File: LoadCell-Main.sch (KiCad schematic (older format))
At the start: 47 parts, among them J1 M20-8760242, J2 0.100_1X4, J3 M20-8760242, J4 0.100_1X4, J5 M20-8760242, J6 0.100_1X4, J7 M20-8760242, J8 0.100_1X4, U1 L78L12ABUTR, U2 LM321SN3T1G, U3 L78L12ABUTR, U4 LM321SN3T1G, U5 L78L12ABUTR, U6 LM321SN3T1G, U7 L78L12ABUTR, U8 LM321SN3T1G

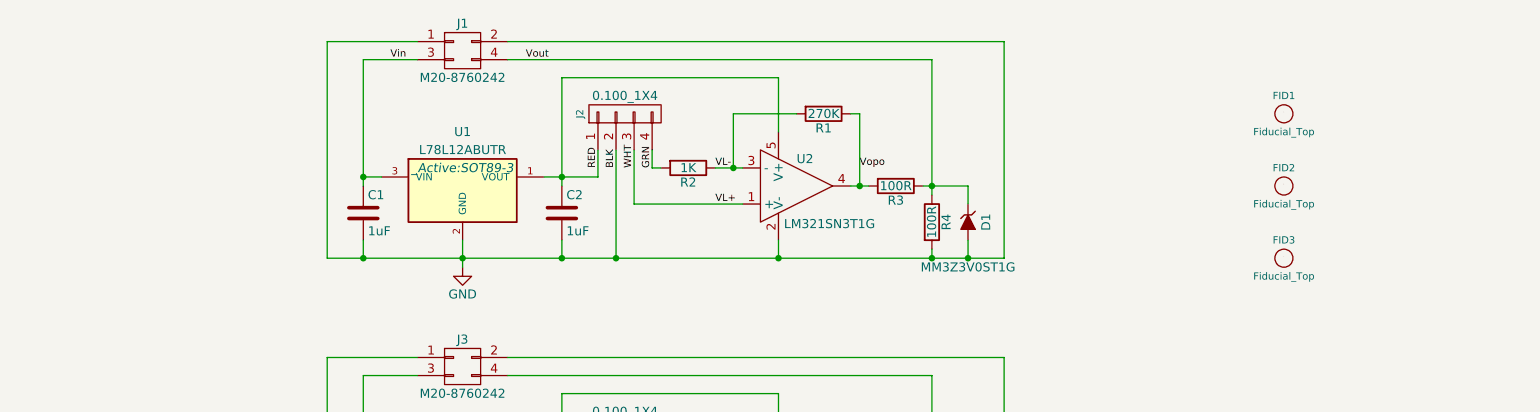
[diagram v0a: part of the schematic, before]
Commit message: Started changes the version 2
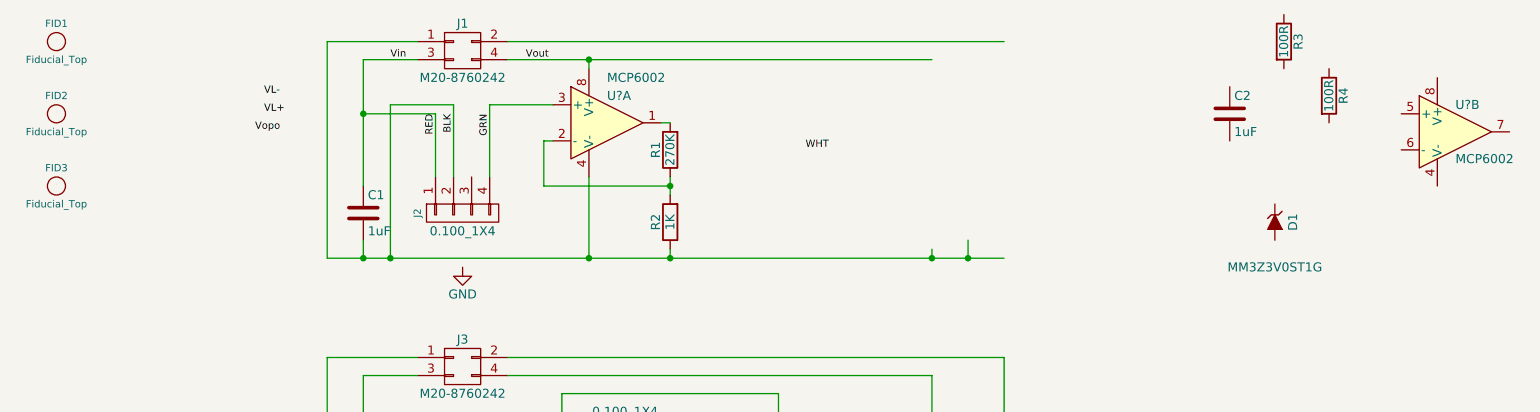
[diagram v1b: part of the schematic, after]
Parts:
- removed U1: L78L12ABUTR, _Active:SOT89-3, symbol L78L12ABUTR
- removed U2: LM321SN3T1G, _Active:SOT-23-5, symbol LM321_23-5
- added U? (x2): MCP6002, symbol MCP6002
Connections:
- wire segments 136 -> 127
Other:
- moved on the sheet: C2, D1, FID1, FID2, FID3, J2, R1, R2, R3, R4
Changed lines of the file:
@@
 L C C2
 U 1 1 5A80CCD0
-P 3850 1750
-F 0 "C2" H 3875 1850 50  0000 L CNN
-F 1 "1uF" H 3875 1650 50  0000 L CNN
-F 2 "_Passive:C_0402" H 3888 1600 50  0001 C CNN
-F 3 "" H 3850 1750 50  0000 C CNN
-	1    3850 1750
+P 7550 1200
+F 0 "C2" H 7575 1300 50  0000 L CNN
+F 1 "1uF" H 7575 1100 50  0000 L CNN
+F 2 "_Passive:C_0402" H 7588 1050 50  0001 C CNN
+F 3 "" H 7550 1200 50  0000 C CNN
+	1    7550 1200
 	1    0    0    -1
 $EndComp
@@
 L R R4
 U 1 1 5A80CD03
-P 5900 1800
-F 0 "R4" V 5980 1800 50  0000 C CNN
-F 1 "100R" V 5900 1800 50  0000 C CNN
-F 2 "_Passive:R_0402" V 5830 1800 50  0001 C CNN
-F 3 "" H 5900 1800 50  0000 C CNN
-	1    5900 1800
-	1    0    0    -1
-$EndComp
-$Comp
-L L78L12ABUTR U1
-U 1 1 5A80CDDA
-P 3300 1600
-F 0 "U1" H 3300 1900 50  0000 C CNN
-F 1 "L78L12ABUTR" H 3300 1800 50  0000 C CNN
-F 2 "_Active:SOT89-3" H 3300 1700 50  0000 C CIN
-F 3 "" H 3300 1600 50  0000 C CNN
-	1    3300 1600
+P 8100 1100
+F 0 "R4" V 8180 1100 50  0000 C CNN
+F 1 "100R" V 8100 1100 50  0000 C CNN
+F 2 "_Passive:R_0402" V 8030 1100 50  0001 C CNN
+F 3 "" H 8100 1100 50  0000 C CNN
+	1    8100 1100
 	1    0    0    -1
 $EndComp
@@
 L R R3
 U 1 1 5A80EB34
-P 5700 1600
-F 0 "R3" V 5780 1600 50  0000 C CNN
-F 1 "100R" V 5700 1600 50  0000 C CNN
-F 2 "_Passive:R_0402" V 5630 1600 50  0001 C CNN
-F 3 "" H 5700 1600 50  0000 C CNN
-	1    5700 1600
-	0    1    1    0
+P 7850 800
+F 0 "R3" V 7930 800 50  0000 C CNN
+F 1 "100R" V 7850 800 50  0000 C CNN
+F 2 "_Passive:R_0402" V 7780 800 50  0001 C CNN
+F 3 "" H 7850 800 50  0000 C CNN
+	1    7850 800
+	1    0    0    -1
 $EndComp
 $Comp
@@
 L R R1
 U 1 1 5A80EC35
-P 5300 1200
-F 0 "R1" V 5380 1200 50  0000 C CNN
-F 1 "270K" V 5300 1200 50  0000 C CNN
-F 2 "_Passive:R_0402" V 5230 1200 50  0001 C CNN
-F 3 "" H 5300 1200 50  0000 C CNN
-	1    5300 1200
-	0    1    1    0
+P 4450 1400
+F 0 "R1" V 4530 1400 50  0000 C CNN
+F 1 "270K" V 4450 1400 50  0000 C CNN
+F 2 "_Passive:R_0402" V 4380 1400 50  0001 C CNN
+F 3 "" H 4450 1400 50  0000 C CNN
+	1    4450 1400
+	-1   0    0    1
 $EndComp
 $Comp
 L R R2
 U 1 1 5A80EC7B
-P 4550 1500
-F 0 "R2" V 4630 1500 50  0000 C CNN
-F 1 "1K" V 4550 1500 50  0000 C CNN
-F 2 "_Passive:R_0402" V 4480 1500 50  0001 C CNN
-F 3 "" H 4550 1500 50  0000 C CNN
-	1    4550 1500
-	0    1    1    0
-$EndComp
-$Comp
-L LM321_23-5 U2
-U 1 1 5A80F3F0
-P 5150 1600
-F 0 "U2" H 5150 1750 50  0000 L CNN
-F 1 "LM321SN3T1G" H 5080 1390 50  0000 L CNN
-F 2 "_Active:SOT-23-5" H 5150 1600 50  0001 C CNN
-F 3 "" H 5150 1600 50  0000 C CNN
-	1    5150 1600
-	1    0    0    -1
+P 4450 1800
+F 0 "R2" V 4530 1800 50  0000 C CNN
+F 1 "1K" V 4450 1800 50  0000 C CNN
+F 2 "_Passive:R_0402" V 4380 1800 50  0001 C CNN
+F 3 "" H 4450 1800 50  0000 C CNN
+	1    4450 1800
+	-1   0    0    1
 $EndComp
 $Comp
 L D_ZENER D1
 U 1 1 5A81D761
-P 6100 1800
-F 0 "D1" H 6100 1900 50  0000 C CNN
-F 1 "MM3Z3V0ST1G" V 6350 1800 50  0000 C CNN
-F 2 "_Passive:SOD-323" H 6100 1800 50  0001 C CNN
-F 3 "" H 6100 1800 50  0000 C CNN
-	1    6100 1800
+P 7800 1800
+F 0 "D1" H 7800 1900 50  0000 C CNN
+F 1 "MM3Z3V0ST1G" V 8050 1800 50  0000 C CNN
+F 2 "_Passive:SOD-323" H 7800 1800 50  0001 C CNN
+F 3 "" H 7800 1800 50  0000 C CNN
+	1    7800 1800
 	0    1    1    0
 $EndComp
@@
 Text Label 3650 900  0    40   ~ 0
 Vout
-Text Label 4700 1500 0    40   ~ 0
+Text Label 2200 1100 0    40   ~ 0
 VL-
-Text Label 4700 1700 0    40   ~ 0
+Text Label 2200 1200 0    40   ~ 0
 VL+
-Text Label 5500 1500 0    40   ~ 0
+Text Label 2150 1300 0    40   ~ 0
 Vopo
 $Comp
 L 0.100_1X4 J2
 U 1 1 5A85E78B
-P 4200 1200
-F 0 "J2" H 4200 1450 40  0000 C CNN
-F 1 "0.100_1X4" V 4300 1200 50  0000 C CNN
-F 2 "_Connector:0.100_1x4_micro" H 4200 1200 50  0001 C CNN
-F 3 "" H 4200 1200 50  0000 C CNN
-	1    4200 1200
-	0    -1   -1   0
-$EndComp
-Text Label 4050 1500 1    40   ~ 0
+P 3300 1750
+F 0 "J2" H 3300 2000 40  0000 C CNN
+F 1 "0.100_1X4" V 3400 1750 50  0000 C CNN
+F 2 "_Connector:0.100_1x4_micro" H 3300 1750 50  0001 C CNN
+F 3 "" H 3300 1750 50  0000 C CNN
+	1    3300 1750
+	0    -1   1    0
+$EndComp
+Text Label 3150 1200 3    40   ~ 0
 RED
-Text Label 4150 1500 1    40   ~ 0
+Text Label 3250 1200 3    40   ~ 0
 BLK
-Text Label 4350 1500 1    40   ~ 0
+Text Label 3450 1200 3    40   ~ 0
 GRN
-Text Label 4250 1500 1    40   ~ 0
+Text Label 5200 1400 0    40   ~ 0
 WHT
 $Comp
@@
 Wire Wire Line
 	2750 900  2750 1600
-Connection ~ 2750 1550
-Wire Wire Line
-	4700 1500 4850 1500
-Wire Wire Line
-	5150 1200 4800 1200
-Wire Wire Line
-	4800 1200 4800 1500
-Connection ~ 4800 1500
-Wire Wire Line
-	5450 1600 5550 1600
-Wire Wire Line
-	5450 1200 5500 1200
-Wire Wire Line
-	5500 1200 5500 1600
-Connection ~ 5500 1600
-Connection ~ 5900 1600
 Connection ~ 5900 2000
 Wire Wire Line
-	5850 1600 6100 1600
-Wire Wire Line
 	2750 1900 2750 2000
 Wire Wire Line
 	5900 2000 5900 1950
 Wire Wire Line
-	6100 1600 6100 1700
-Wire Wire Line
 	6100 2000 6100 1900
 Wire Wire Line
 	3050 900  2750 900
 Wire Wire Line
-	2850 1550 2750 1550
-Wire Wire Line
 	2550 800  3050 800
-Wire Wire Line
-	3750 1550 4050 1550
-Connection ~ 3850 1550
-Wire Wire Line
-	3850 2000 3850 1900
-Wire Wire Line
-	4050 1550 4050 1400
-Wire Wire Line
-	3850 1000 3850 1600
-Wire Wire Line
-	4150 2000 4150 1400
-Wire Wire Line
-	3850 1000 5050 1000
-Wire Wire Line
-	5050 1000 5050 1300
-Wire Wire Line
-	4350 1400 4350 1500
-Wire Wire Line
-	4350 1500 4400 1500
-Wire Wire Line
-	4850 1700 4250 1700
-Wire Wire Line
-	4250 1700 4250 1400
 Wire Wire Line
 	2550 2000 6300 2000
 Connection ~ 2750 2000
 Wire Wire Line
-	3300 1900 3300 2050
-Connection ~ 3300 2000
-Connection ~ 3850 2000
-Connection ~ 4150 2000
-Wire Wire Line
-	5050 1900 5050 2000
-Connection ~ 5050 2000
-Wire Wire Line
 	3550 900  5900 900
-Wire Wire Line
-	5900 900  5900 1650
 Wire Wire Line
 	3550 800  6300 800
@@
 Wire Wire Line
 	5900 6350 5900 7100
-Wire Wire Line
-	6300 800  6300 2000
 Connection ~ 6100 2000
 Wire Wire Line
@@
 L Fiducial_Top FID1
 U 1 1 5A8C10DE
-P 7850 1200
-F 0 "FID1" H 7850 1300 40  0000 C CNN
-F 1 "Fiducial_Top" H 7850 1100 40  0000 C CNN
-F 2 "_Connector:Fiducial_0.040_Top" H 7850 1200 150 0001 C CNN
-F 3 "" H 7850 1200 150 0000 C CNN
-	1    7850 1200
+P 1050 800
+F 0 "FID1" H 1050 900 40  0000 C CNN
+F 1 "Fiducial_Top" H 1050 700 40  0000 C CNN
+F 2 "_Connector:Fiducial_0.040_Top" H 1050 800 150 0001 C CNN
+F 3 "" H 1050 800 150 0000 C CNN
+	1    1050 800
 	1    0    0    -1
 $EndComp
@@
 L Fiducial_Top FID2
 U 1 1 5A8C1162
-P 7850 1600
-F 0 "FID2" H 7850 1700 40  0000 C CNN
-F 1 "Fiducial_Top" H 7850 1500 40  0000 C CNN
-F 2 "_Connector:Fiducial_0.040_Top" H 7850 1600 150 0001 C CNN
-F 3 "" H 7850 1600 150 0000 C CNN
-	1    7850 1600
+P 1050 1200
+F 0 "FID2" H 1050 1300 40  0000 C CNN
+F 1 "Fiducial_Top" H 1050 1100 40  0000 C CNN
+F 2 "_Connector:Fiducial_0.040_Top" H 1050 1200 150 0001 C CNN
+F 3 "" H 1050 1200 150 0000 C CNN
+	1    1050 1200
 	1    0    0    -1
 $EndComp
@@
 L Fiducial_Top FID3
 U 1 1 5A8C11D3
-P 7850 2000
-F 0 "FID3" H 7850 2100 40  0000 C CNN
-F 1 "Fiducial_Top" H 7850 1900 40  0000 C CNN
-F 2 "_Connector:Fiducial_0.040_Top" H 7850 2000 150 0001 C CNN
-F 3 "" H 7850 2000 150 0000 C CNN
-	1    7850 2000
-	1    0    0    -1
-$EndComp
+P 1050 1600
+F 0 "FID3" H 1050 1700 40  0000 C CNN
+F 1 "Fiducial_Top" H 1050 1500 40  0000 C CNN
+F 2 "_Connector:Fiducial_0.040_Top" H 1050 1600 150 0001 C CNN
+F 3 "" H 1050 1600 150 0000 C CNN
+	1    1050 1600
+	1    0    0    -1
+$EndComp
+$Comp
+L MCP6002 U?
+U 1 1 5ADCF38B
+P 4100 1250
+F 0 "U?" H 4100 1400 50  0000 L CNN
+F 1 "MCP6002" H 4100 1500 50  0000 L CNN
+F 2 "" H 4000 1300 50  0000 C CNN
+F 3 "" H 4100 1400 50  0000 C CNN
+	1    4100 1250
+	1    0    0    -1
+$EndComp
+$Comp
+L MCP6002 U?
+U 2 1 5ADCF54D
+P 8800 1300
+F 0 "U?" H 8800 1450 50  0000 L CNN
+F 1 "MCP6002" H 8800 1150 50  0000 L CNN
+F 2 "" H 8700 1350 50  0000 C CNN
+F 3 "" H 8800 1450 50  0000 C CNN
+	2    8800 1300
+	1    0    0    -1
+$EndComp
+Wire Wire Line
+	3150 1200 3150 1550
+Wire Wire Line
+	2750 1200 3150 1200
+Connection ~ 2750 1200
+Wire Wire Line
+	3250 1150 3250 1550
+Wire Wire Line
+	2900 1150 3250 1150
+Wire Wire Line
+	2900 1150 2900 2000
+Connection ~ 2900 2000
+Wire Wire Line
+	4000 950  4000 900
+Connection ~ 4000 900
+Wire Wire Line
+	4000 1550 4000 2000
+Connection ~ 4000 2000
+Wire Wire Line
+	4400 1250 4450 1250
+Wire Wire Line
+	4450 1550 4450 1650
+Wire Wire Line
+	4450 1950 4450 2000
+Connection ~ 4450 2000
+Wire Wire Line
+	3800 1350 3750 1350
+Wire Wire Line
+	3750 1350 3750 1600
+Wire Wire Line
+	3750 1600 4450 1600
+Connection ~ 4450 1600
+Wire Wire Line
+	3450 1550 3450 1150
+Wire Wire Line
+	3450 1150 3800 1150
 $EndSCHEMATC
